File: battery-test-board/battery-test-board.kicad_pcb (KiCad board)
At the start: 2 copper layers, 118.9 x 134.4 mm, 58 parts, among them J1 Conn_02x04_Odd_Even, J10 Screw_Terminal_01x02, J2 Conn_02x04_Odd_Even, J3 Screw_Terminal_01x02, J4 Screw_Terminal_01x02, J5 Screw_Terminal_01x02, J6 Screw_Terminal_01x02, J7 Conn_02x04_Odd_Even, J8 Conn_02x20_Odd_Even, J9 Conn_02x20_Odd_Even, Q1 PJA3412-AU_R1_000A1, Q2 PJA3412-AU_R1_000A1, U1 J104D2C12VDC.15S‎, U10 J104D2C12VDC.15S‎, U2 J104D2C12VDC.15S‎, U3 J104D2C12VDC.15S‎, U4 J104D2C12VDC.15S‎, U5 J104D2C12VDC.15S‎, U6 J104D2C12VDC.15S‎, U7 J104D2C12VDC.15S‎, U8 J104D2C12VDC.15S‎, U9 J104D2C12VDC.15S‎

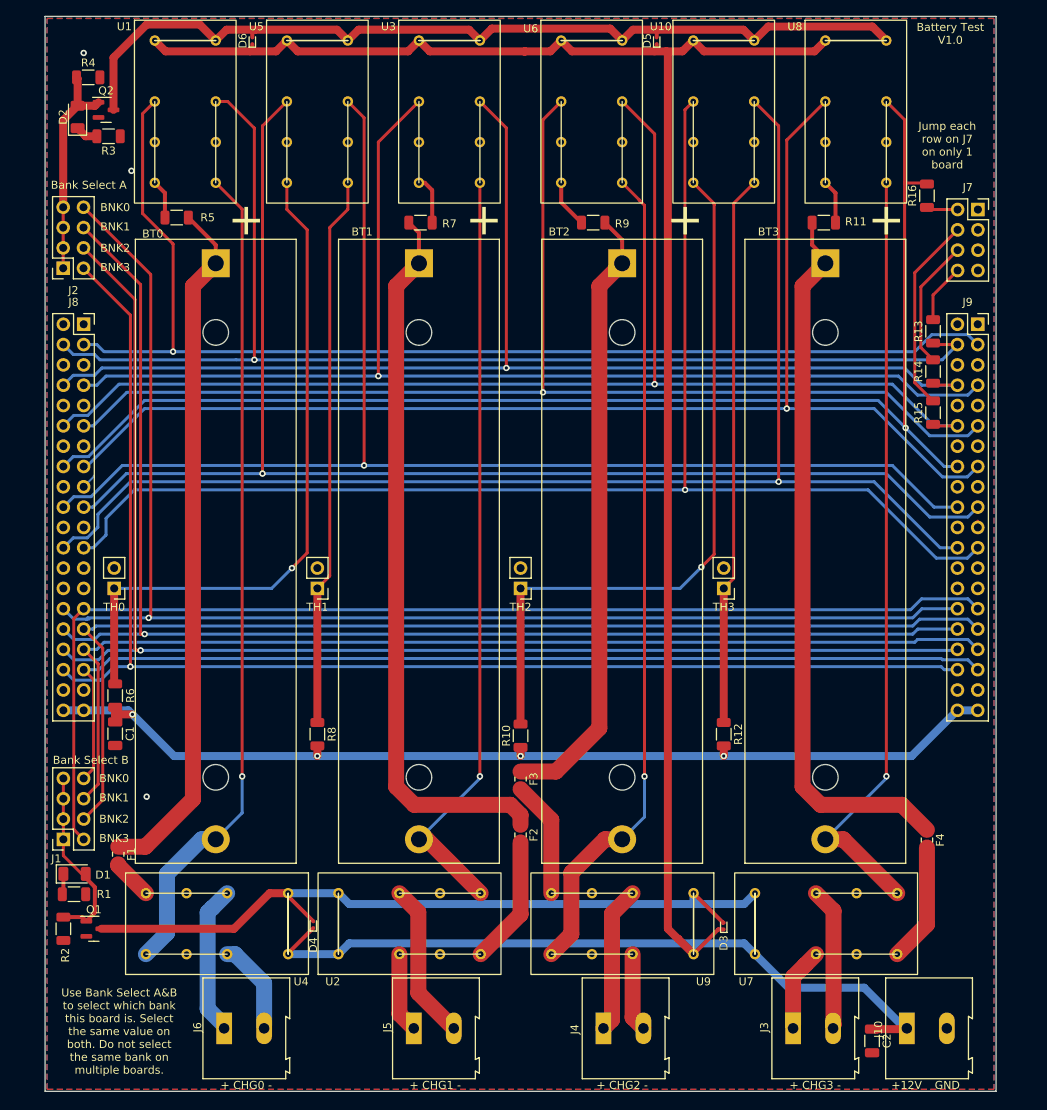
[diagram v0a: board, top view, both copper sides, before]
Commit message: Updated footprints and PCB
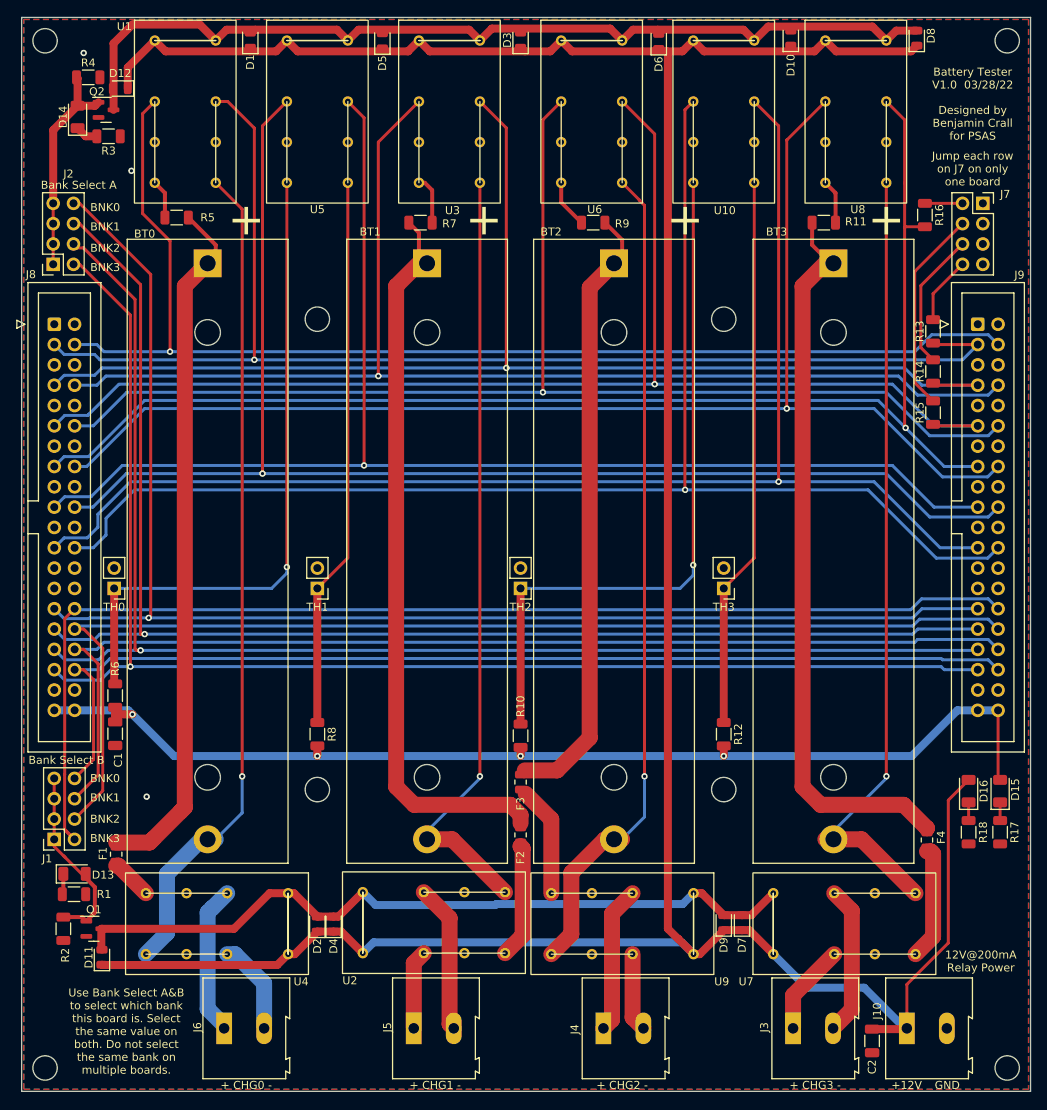
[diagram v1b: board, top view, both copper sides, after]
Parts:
- added D1: diode, Diode_SMD:D_0805_2012Metric, F.Cu at (56.4, 28.6)
- added D10: diode, Diode_SMD:D_0805_2012Metric, F.Cu at (124.0, 28.4)
- added D15: Green, LED_SMD:LED_1206_3216Metric, F.Cu at (150.1, 122.5)
- added D16: Green, LED_SMD:LED_1206_3216Metric, F.Cu at (146.2, 122.5)
- added D2: diode, Diode_SMD:D_0805_2012Metric, F.Cu at (64.8, 139.1)
- added D4: diode, Diode_SMD:D_0805_2012Metric, F.Cu at (66.8, 139.1)
- added D5: diode, Diode_SMD:D_0805_2012Metric, F.Cu at (72.9, 28.7)
- added D7: diode, Diode_SMD:D_0805_2012Metric, F.Cu at (117.9, 138.9)
- added D8: diode, Diode_SMD:D_0805_2012Metric, F.Cu at (139.7, 28.4)
- added D9: diode, Diode_SMD:D_0805_2012Metric, F.Cu at (115.6, 138.9)
- added R17: 4k7, Resistor_SMD:R_1206_3216Metric, F.Cu at (150.1, 127.6)
- added R18: 10k, Resistor_SMD:R_1206_3216Metric, F.Cu at (146.2, 127.6)
- added REF**: MountingHole_3mm, MountingHole:MountingHole_3mm, F.Cu at (115.6, 122.3)
- added REF**: MountingHole_3mm, MountingHole:MountingHole_3mm, F.Cu at (30.7, 157.1)
- added REF**: MountingHole_3mm, MountingHole:MountingHole_3mm, F.Cu at (151.0, 28.7)
- added REF**: MountingHole_3mm, MountingHole:MountingHole_3mm, F.Cu at (64.8, 63.5)
- added REF**: MountingHole_3mm, MountingHole:MountingHole_3mm, F.Cu at (64.8, 122.3)
- added REF**: MountingHole_3mm, MountingHole:MountingHole_3mm, F.Cu at (151.0, 157.1)
- added REF**: MountingHole_3mm, MountingHole:MountingHole_3mm, F.Cu at (115.6, 63.5)
- added REF**: MountingHole_3mm, MountingHole:MountingHole_3mm, F.Cu at (30.7, 28.7)
- BT0, BT1, BT2, BT3: value BK-18650-PC2 -> battery
- C1, C2: value C -> 10u
- D11: renamed from D4; value D -> diode; footprint Diode_SMD:D_SOD-923 -> Diode_SMD:D_0805_2012Metric
- D12: renamed from D5; value D -> diode; footprint Diode_SMD:D_SOD-923 -> Diode_SMD:D_0805_2012Metric
- D13: renamed from D1; value LED -> Amber
- D14: renamed from D2; value LED -> Amber
- D3, D6: value D -> diode; footprint Diode_SMD:D_SOD-923 -> Diode_SMD:D_0805_2012Metric
- J8, J9: value Conn_02x20_Odd_Even -> connector; footprint Connector_PinSocket_2.54mm:PinSocket_2x20_P2.54mm_Vertical -> Connector_IDC:IDC-Header_2x20_P2.54mm_Vertical
- Q1, Q2: value PJA3412-AU_R1_000A1 -> mosfet
- R1, R3: value 330 -> 4k7
- R11, R5, R7, R9: value 1k -> 470
- U1, U10, U2, U3, U4, U5, U6, U7, U8, U9: value J104D2C12VDC.15S‎ -> relay
- moved D3 113.6 mm to (90.2, 28.6)
- moved D12 67.3 mm to (40.1, 34.7), turned to 180 degrees
- moved D6 50.8 mm to (107.4, 28.8)
- moved D11 26.7 mm to (37.8, 143.3)
- moved J8 3.67 mm to (31.9, 64.1)
- moved U4 3.05 mm to (65.4, 137.7)
- moved R16 2.43 mm to (140.7, 50.5), turned to -90 degrees
- moved U9 2.29 mm to (116.7, 137.8)
- moved J2 1.34 mm to (31.8, 56.6)
- moved J1 1.14 mm to (31.9, 128.5)
- moved BT1 1.02 mm to (78.5, 56.5)
- moved BT2 1.02 mm to (101.9, 56.5)
- moved BT0 1.02 mm to (51.1, 56.5)
- moved BT3 1.02 mm to (129.3, 56.5)
- moved J7 0.99 mm to (148.0, 49.0)
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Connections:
- D3 pad 2: relay_c -> relay_v
- J8 pad 11: batt_2+ -> batt_2-
- J8 pad 12: batt_2- -> batt_2+
- J8 pad 15: batt_3+ -> batt_3-
- J8 pad 16: batt_3- -> batt_3+
- J8 pad 19: batt_0t -> batt_1t
- J8 pad 20: batt_1t -> batt_0t
- J8 pad 23: batt_2t -> batt_3t
- J8 pad 24: batt_3t -> batt_2t
- J8 pad 29: bank_0c -> bank_0m
- J8 pad 3: batt_0+ -> batt_0-
- J8 pad 30: bank_0m -> bank_0c
- J8 pad 31: bank_1c -> bank_1m
- J8 pad 32: bank_1m -> bank_1c
- J8 pad 33: bank_2c -> bank_2m
- J8 pad 34: bank_2m -> bank_2c
- J8 pad 35: bank_3c -> bank_3m
- J8 pad 36: bank_3m -> bank_3c
- J8 pad 4: batt_0- -> batt_0+
- J8 pad 7: batt_1+ -> batt_1-
- J8 pad 8: batt_1- -> batt_1+
- J9 pad 11: batt_2+ -> batt_2-
- J9 pad 12: batt_2- -> batt_2+
- J9 pad 15: batt_3+ -> batt_3-
- J9 pad 16: batt_3- -> batt_3+
- J9 pad 19: batt_0t -> batt_1t
- J9 pad 20: batt_1t -> batt_0t
- J9 pad 23: batt_2t -> batt_3t
- J9 pad 24: batt_3t -> batt_2t
- J9 pad 29: bank_0c -> bank_0m
- J9 pad 3: batt_0+ -> batt_0-
- J9 pad 30: bank_0m -> bank_0c
- J9 pad 31: bank_1c -> bank_1m
- J9 pad 32: bank_1m -> bank_1c
- J9 pad 33: bank_2c -> bank_2m
- J9 pad 34: bank_2m -> bank_2c
- J9 pad 35: bank_3c -> bank_3m
- J9 pad 36: bank_3m -> bank_3c
- J9 pad 4: batt_0- -> batt_0+
- J9 pad 7: batt_1+ -> batt_1-
- J9 pad 8: batt_1- -> batt_1+
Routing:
- net +12V: track 303.3 -> 372.9 mm
- net +5V: track 126.6 -> 138.4 mm
- net batt_2-: track 156.2 -> 162.7 mm
- net batt_1-: track 151.4 -> 157.6 mm
- net batt_0-: track 151.6 -> 157.8 mm
- net bank_0c: track 142.7 -> 148.0 mm
- net bank_3m: track 165.4 -> 170.5 mm
- net bank_1m: track 167.1 -> 172.2 mm
- net bank_2m: track 166.4 -> 171.5 mm
- net bank_2c: track 133.0 -> 138.1 mm
- net bank_1c: track 138.5 -> 143.6 mm
- net bank_3c: track 127.5 -> 132.6 mm
- net bank_0m: track 168.0 -> 172.7 mm
- net batt_3t: track 168.3 -> 172.0 mm
- net batt_1t: track 162.4 -> 166.1 mm
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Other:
- board size 118.9 x 134.4 mm -> 126.1 x 134.2 mm
- board text added: "12V@200mA Relay Power"
- board text added: "Battery Tester V1.0 03/28/22"
- board text added: "Designed by Benjamin Crall for PSAS"
- board text added: "Jump each row on J7 on only one board"
- board text added: "TODO fix spacing between pads"
- board text removed: "Battery Test V1.0"
- board text removed: "Jump each row on J7 on only 1 board"
